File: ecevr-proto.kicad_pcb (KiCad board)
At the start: 4 copper layers, 100 x 92 mm, 359 parts, among them J1 CUR_SEL, J19 SFP, J2 PEN_SEL, J20 SFP_CAGE, J2001 BNC, J2051 BNC, J2201 BEL_0845_2G1T_H5, J3 USB_C_Receptacle_USB2.0, J4 JTAG, Q1 SSM6N35AFE, Q2 SSM6N35AFE, Q3 Si3477, SW1 PROG, SW2101 SW_DIP_x08, U1 XC7A35T-CSG325, U10 74VHC1G03, U11 UTC2000, U12 5P49V6965, U13 TPS3808DBV, U14 74LVC1G06, U15 74LVC2T45DC, U16 74LVC2T45DC, U2 AT25SL641, U2001 74LVC2T45DC, U2051 74LVC2T45DC, U2101 74AHC1T86, U2102 74AHC1T86, U2103 PCA9306, U2104 24AA0x, U2105 74AHC1T86, U2106 74AHC1T86, U2201 74AHC1T86, U2202 74LVC1G06, U2301 lan9254, U2302 SN74LV1T34DBV, U3 FT240XQ, U4 TLV62569ADDC, U5 TPS62A01A-SOT563, U6 TPS62A01A-SOT563, U7 TLV62569ADDC, U8 74ALVC125, U9 TLV62569ADDC, X2301 FNETHE025, Y1 25MHz

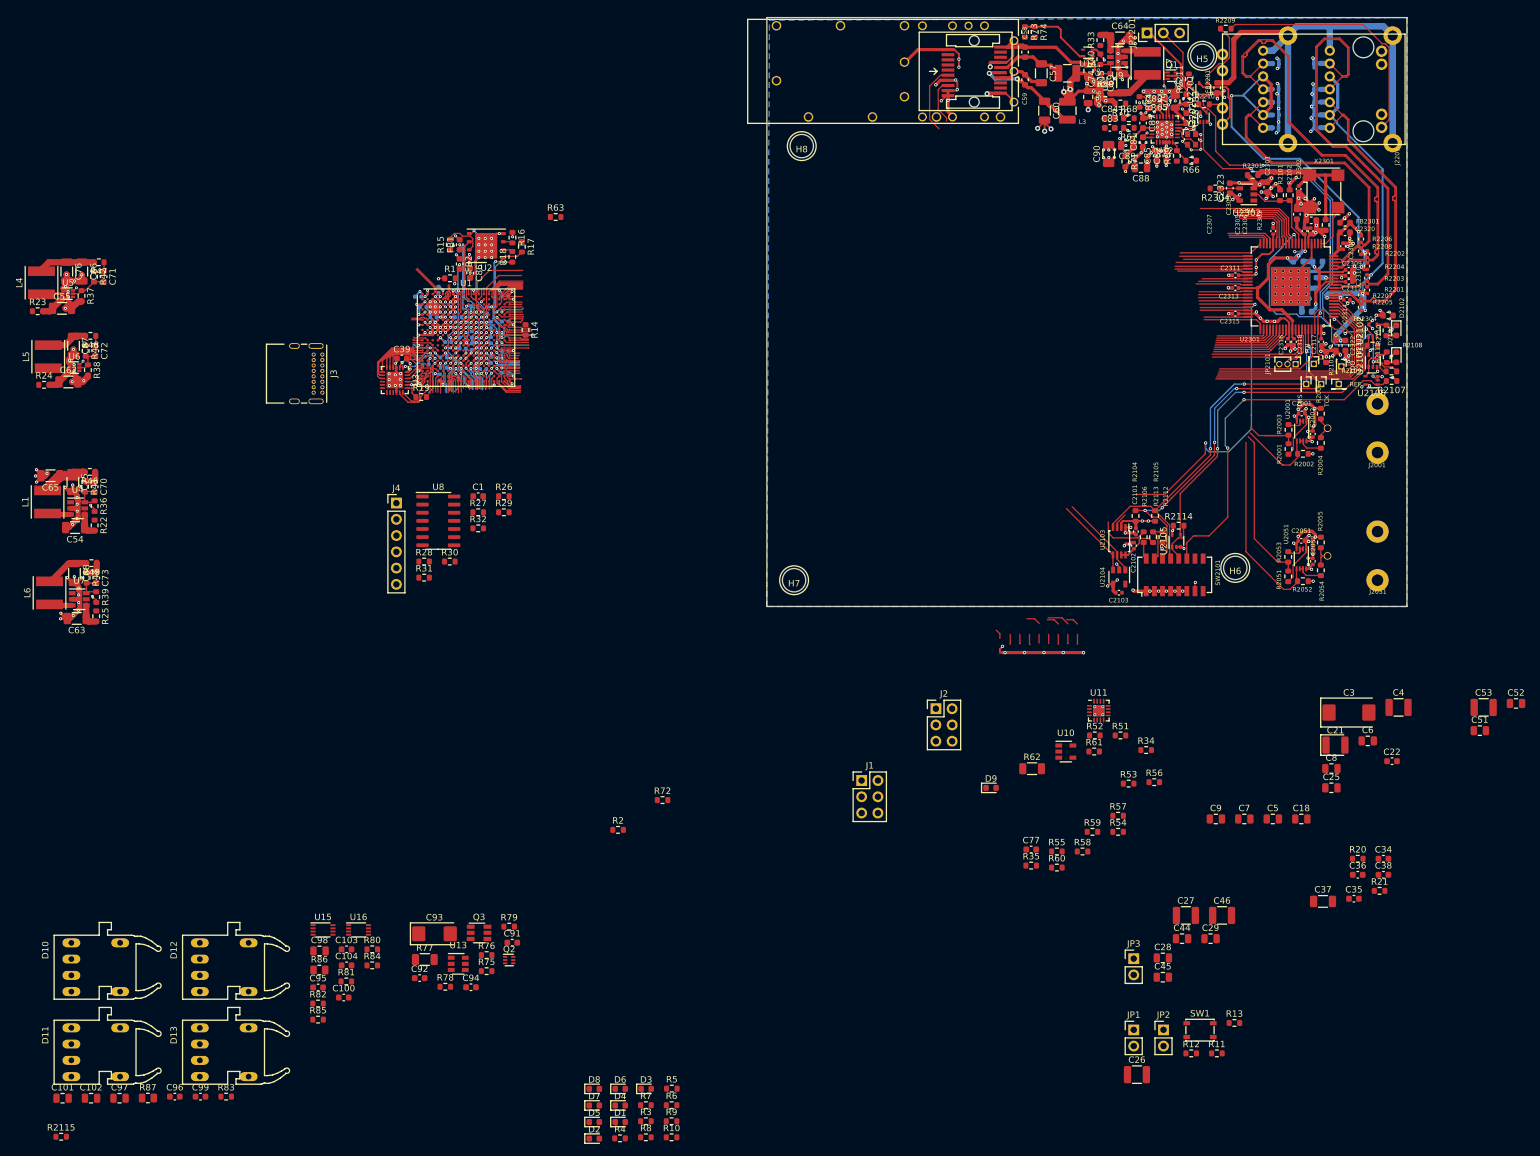
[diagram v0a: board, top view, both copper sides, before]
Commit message: further work...
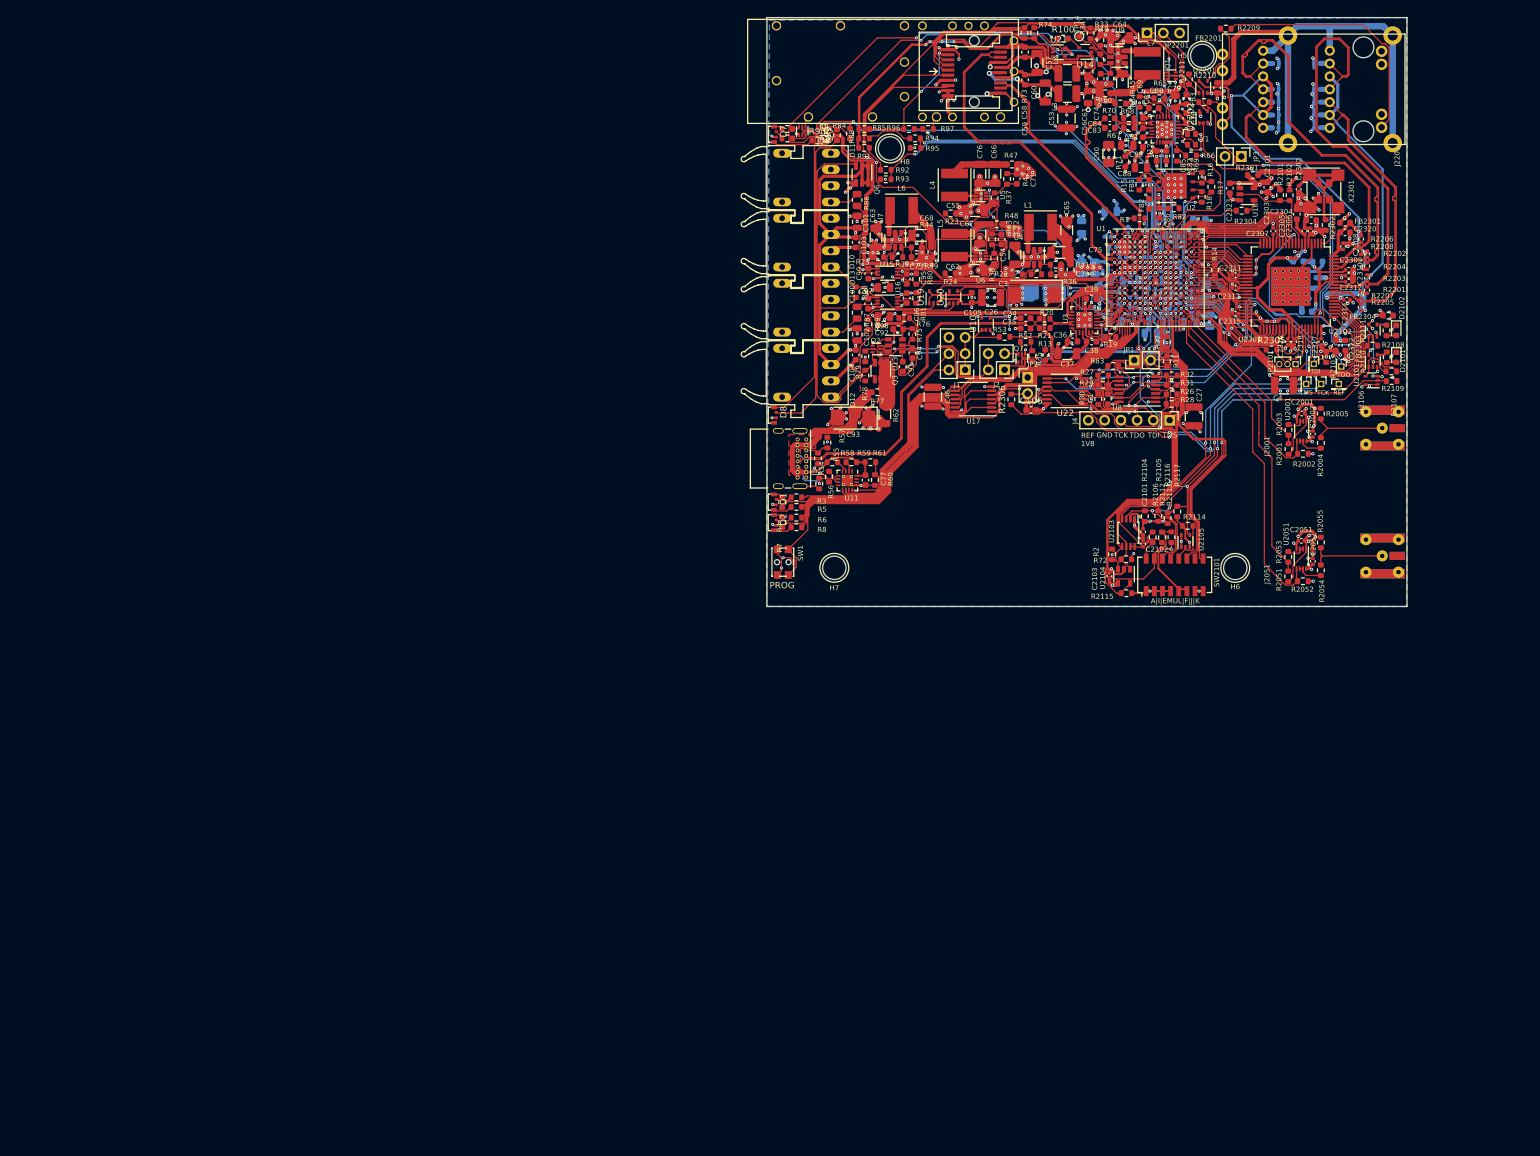
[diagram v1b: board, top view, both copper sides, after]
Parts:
- removed D3, D4, D5, D6, D9: LED, LED_SMD:LED_0603_1608Metric
- removed R51: 1k, Resistor_SMD:R_0603_1608Metric
- removed R63: 4k7, Resistor_SMD:R_0603_1608Metric
- removed U2302: SN74LV1T34DBV, Package_TO_SOT_SMD:SOT-23-5
- added C105: 100nF, Capacitor_SMD:C_0603_1608Metric, F.Cu at (132.0, 73.8)
- added C106: 100nF_603, Capacitor_SMD:C_0603_1608Metric, F.Cu at (141.3, 91.3)
- added Q4: SSM6N35AFE, proj_footprints:SOT-563-adjusted, F.Cu at (108.9, 47.5)
- added Q5: SSM6N35AFE, proj_footprints:SOT-563-adjusted, F.Cu at (105.5, 47.7)
- added Q6: Si3477, Package_TO_SOT_SMD:TSOT-23-6, F.Cu at (114.9, 54.5)
- added Q7: SSM6N35AFE, proj_footprints:SOT-563-adjusted, F.Cu at (139.8, 83.2)
- added R100: 2k, Resistor_SMD:R_0603_1608Metric, F.Cu at (146.3, 33.3)
- added R2116: 0, Resistor_SMD:R_0603_1608Metric, F.Cu at (162.6, 108.2)
- added R2117: 0, Resistor_SMD:R_0603_1608Metric, F.Cu at (164.1, 107.2)
- added R2305: 0, Resistor_SMD:R_0603_1608Metric, F.Cu at (178.8, 81.8)
- added R2306: 10k, Resistor_SMD:R_0603_1608Metric, F.Cu at (138.2, 89.7)
- added R88: 4k7, Resistor_SMD:R_0603_1608Metric, F.Cu at (115.2, 48.9)
- added R89: 1k, Resistor_SMD:R_0603_1608Metric, F.Cu at (115.8, 77.9)
- added R90: 1k, Resistor_SMD:R_0603_1608Metric, F.Cu at (113.9, 72.9)
- added R91: 4k7, Resistor_SMD:R_0603_1608Metric, F.Cu at (115.2, 50.4)
- added R92: 47k, Resistor_SMD:R_0603_1608Metric, F.Cu at (118.6, 53.8)
- added R93: 47k, Resistor_SMD:R_0603_1608Metric, F.Cu at (118.6, 55.3)
- added R94: 47k, Resistor_SMD:R_0603_1608Metric, F.Cu at (123.2, 48.9)
- added R95: 47k, Resistor_SMD:R_0603_1608Metric, F.Cu at (123.2, 50.4)
- added R96: 47k, Resistor_SMD:R_0603_1608Metric, F.Cu at (122.2, 47.4)
- added R97: 47k, Resistor_SMD:R_0603_1608Metric, F.Cu at (125.2, 47.4)
- added R98: 230, Resistor_SMD:R_0603_1608Metric, F.Cu at (107.9, 49.2)
- added R99: 750, Resistor_SMD:R_0603_1608Metric, F.Cu at (110.9, 48.4)
- added TP1: Dummy End, proj_footprints:endpoint_0.1mm, B.Cu at (162.8, 62.8)
- added TP10: Dummy End, proj_footprints:endpoint_0.1mm, F.Cu at (155.1, 79.4)
- added TP11: Dummy End, proj_footprints:endpoint_0.1mm, B.Cu at (157.5, 79.0)
- added TP12: Dummy End, proj_footprints:endpoint_0.1mm, B.Cu at (157.7, 79.0)
- added TP13: Dummy End, proj_footprints:endpoint_0.1mm, B.Cu at (157.9, 79.0)
- added TP14: TestPoint, TestPoint:TestPoint_Pad_D1.0mm, F.Cu at (148.8, 32.9)
- added TP2: Dummy End, proj_footprints:endpoint_0.1mm, F.Cu at (163.1, 62.8)
- added TP3: Dummy End, proj_footprints:endpoint_0.1mm, B.Cu at (164.8, 62.3)
- added TP4: Dummy End, proj_footprints:endpoint_0.1mm, B.Cu at (164.4, 79.0)
- added TP5: Dummy End, proj_footprints:endpoint_0.1mm, F.Cu at (164.8, 79.0)
- added TP6: Dummy End, proj_footprints:endpoint_0.1mm, B.Cu at (163.9, 79.0)
- added TP7: Dummy End, proj_footprints:endpoint_0.1mm, F.Cu at (163.9, 79.0)
- added TP8: Dummy End, proj_footprints:endpoint_0.1mm, F.Cu at (164.3, 79.0)
- added U17: 74LVC06, Package_SO:TSSOP-14_4.4x5mm_P0.65mm, F.Cu at (132.3, 89.6)
- added U18: 74LVC1T126, Package_TO_SOT_SMD:SOT-23-5, F.Cu at (175.0, 57.6)
- added U19: 74AHC1T86, Package_TO_SOT_SMD:SOT-353_SC-70-5, F.Cu at (126.0, 73.7)
- added U20: 74AHC1T86, Package_TO_SOT_SMD:SOT-353_SC-70-5, F.Cu at (129.1, 73.7)
- added U21: 74LVC1G06, Package_TO_SOT_SMD:SOT-353_SC-70-5, F.Cu at (145.6, 35.4)
- added U22: 74AC126, Package_SO:TSSOP-14_4.4x5mm_P0.65mm, F.Cu at (146.6, 88.3)
- C18, C21, C25, C28, C29, C44, C45, C5, C51, C52, C6, C7, C8, C9: moved to B.Cu
- C22: footprint Capacitor_SMD:C_0603_1608Metric -> Capacitor_SMD:C_0402_1005Metric; moved to B.Cu
- D1, D2, D7, D8: value LED -> LED_BARG; footprint LED_SMD:LED_0603_1608Metric -> proj_footprints:LED_RGB_2504_horiz_barg
- J2: footprint Connector_PinHeader_2.54mm:PinHeader_2x03_P2.54mm_Vertical -> Connector_PinHeader_2.54mm:PinHeader_2x02_P2.54mm_Vertical
- J2001, J2051: footprint proj_footprints:BNC_Molex_0731713150 -> proj_footprints:LEMO+SMA
- R10, R3, R6: value 1k -> 750
- R15, R16, R17: value 2k4 -> 10k
- R2002, R2052: value 2k2 -> 3k3
- R2108: value 1k -> 10k
- R2110: value 100 -> 1k5
- R2111: value 100 -> 3k3
- R22, R23, R24, R25, R33: value 10k -> 100k
- R2209, R2210: value 100 -> 178
- R2211: value 100 -> 10k
- R4, R7, R9: value 1k -> 2k
- R40: value 45.9k -> 10k
- R45: value 10.2k -> 45k3
- R5, R8: value 1k -> 230
- R52, R76: value 100k -> 10k
- R66: value 1k78 -> 10k
- R75: value 100k -> 45.3k
- R77: value 47 -> 50; footprint Resistor_SMD:R_1206_3216Metric -> Resistor_SMD:R_0603_1608Metric
- R82, R83: value 1k -> 100k
- R84, R85: value 1k -> 4k7
- R86, R87: value 90 -> 100
- SW1: footprint Button_Switch_SMD:SW_SPST_PTS810 -> proj_footprints:SW_SPST_PTS810_and_PTS841
- U10: value 74VHC1G03 -> 74LVC1G06; footprint Package_TO_SOT_SMD:SOT-23-5 -> Package_TO_SOT_SMD:SOT-353_SC-70-5
- U14, U2202: footprint proj_footprints:SOT-5x3 -> Package_TO_SOT_SMD:SOT-353_SC-70-5
- U2104: value 24AA0x -> 24FC16T
- U8: footprint Package_SO:SOIC-14_3.9x8.7mm_P1.27mm -> Package_SO:TSSOP-14_4.4x5mm_P0.65mm
- X2301: footprint Oscillator:Oscillator_SMD_Diodes_FN-4Pin_7.0x5.0mm -> proj_footprints:FNETH_and_ASE-4Pin_3.2x2.5mm
- moved R2115 186.8 mm to (156.2, 119.9)
- moved C101 184.8 mm to (114.1, 61.9), turned to 90 degrees
- moved R82 182.5 mm to (163.6, 59.8)
- moved D11 181.0 mm to (110.0, 55.0), turned to 180 degrees
- moved R83 179.5 mm to (154.1, 84.4)
- moved C97 174.1 mm to (118.3, 72.2)
- moved C96 169.2 mm to (121.8, 73.8), turned to 90 degrees
- moved C102 169.0 mm to (114.1, 79.5), turned to 90 degrees
- moved C99 165.6 mm to (115.8, 70.0), turned to 90 degrees
- moved R87 165.3 mm to (114.1, 76.1), turned to 270 degrees
- moved D10 164.0 mm to (110.0, 65.2), turned to 180 degrees
- moved C65 163.3 mm to (146.8, 63.2), turned to 90 degrees
- moved R85 163.2 mm to (115.2, 47.4), turned to 180 degrees
- moved L1 161.0 mm to (142.8, 62.8), turned to 0 degrees
- moved C75 158.4 mm to (145.9, 66.7), turned to 180 degrees
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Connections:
- C101 pad 1: +5V -> +5V_SWITCHED
- C102 pad 1: +5V -> +5V_SWITCHED
- C103 pad 2: +5V -> +5V_SWITCHED
- C104 pad 2: +5V -> +5V_SWITCHED
- D1 pad 1: GND -> Net-(D1-Pad1)
- D1 pad 2: Net-(D1-Pad2) -> +5V
- D10 pad 3: +5V -> +5V_SWITCHED
- D12 pad 3: +5V -> +5V_SWITCHED
- D2 pad 1: GND -> Net-(D2-Pad1)
- D2 pad 2: Net-(D2-Pad2) -> +5V
- D7 pad 1: GND -> Net-(D7-Pad1)
- D7 pad 2: Net-(D7-Pad2) -> +5V
- D8 pad 1: GND -> Net-(D8-Pad1)
- D8 pad 2: Net-(D8-Pad2) -> +5V
- J19 pad 2: IO_L7N_T1_AD2N_15 -> Net-(J19-Pad2)
- J19 pad 6: IO_L5N_T0_AD9N_15 -> Net-(J19-Pad6)
- J19 pad 8: IO_L4N_T0_15 -> Net-(J19-Pad8)
- J2 pad 2: USB_BCDb -> Net-(J2-Pad2)
- J2 pad 3: Net-(J2-Pad1) -> Net-(J2-Pad3)
- J2 pad 4: IO_L15N_T2_DQS_34 -> Net-(J2-Pad2)
- Q1 pad 1: IO_L7P_T1_AD2P_15 -> IO_L4N_T0_15
- Q2 pad 3: Net-(Q2-Pad3) -> Net-(J2-Pad2)
- R10 pad 1: IO_L20P_T3_34 -> Net-(D7-Pad3)
- R10 pad 2: Net-(D8-Pad2) -> Net-(Q5-Pad3)
- R2 pad 2: IO_L23N_T3_A02_D18_14 -> IO_L23P_T3_A03_D19_14
- R2107 pad 1: +3V3 -> GND
- R2108 pad 2: Net-(R2108-Pad2) -> IO_L22P_T3_A05_D21_14
- R2112 pad 1: IO_L21P_T3_DQS_14 -> IO_L23N_T3_A02_D18_14
- R2113 pad 2: IO_L21P_T3_DQS_14 -> IO_L23N_T3_A02_D18_14
- R2114 pad 1: +1V8 -> GND
- R2114 pad 2: IO_L22P_T3_A05_D21_14 -> Net-(R2114-Pad2)
- R3 pad 1: IO_L3P_T0_DQS_34 -> Net-(R3-Pad1)
- R3 pad 2: Net-(D1-Pad2) -> Net-(D1-Pad3)
- R35 pad 1: Net-(R35-Pad1) -> USB_BCDb
- R35 pad 2: +5V -> GND
- R4 pad 1: IO_L3N_T0_DQS_34 -> Net-(R4-Pad1)
- R4 pad 2: Net-(D2-Pad2) -> Net-(D1-Pad4)
- R5 pad 1: IO_L18N_T2_34 -> Net-(R5-Pad1)
- R5 pad 2: Net-(D3-Pad2) -> Net-(D1-Pad1)
- R52 pad 1: Net-(J2-Pad1) -> IO_L15N_T2_DQS_34
- R52 pad 2: +5V -> GND
- R6 pad 1: IO_L18P_T2_34 -> Net-(R6-Pad1)
- R6 pad 2: Net-(D4-Pad2) -> Net-(D2-Pad3)
- R64 pad 1: IO_L7P_T1_AD2P_15 -> IO_L4N_T0_15
- R7 pad 1: IO_25_34 -> Net-(R7-Pad1)
- R7 pad 2: Net-(D5-Pad2) -> Net-(D2-Pad4)
- R72 pad 2: IO_L23P_T3_A03_D19_14 -> IO_L21P_T3_DQS_14
- R8 pad 1: IO_L20N_T3_34 -> Net-(R8-Pad1)
- R8 pad 2: Net-(D6-Pad2) -> Net-(D2-Pad1)
- R80 pad 1: IO_L22P_T3_34 -> IO_L4P_T0_34
- R81 pad 1: IO_L22N_T3_34 -> IO_L4N_T0_34
- R82 pad 1: IO_L24N_T3_34 -> +1V8
- R82 pad 2: GND -> Net-(R82-Pad2)
- R83 pad 1: IO_L24P_T3_34 -> +1V8
- R83 pad 2: GND -> TDO
- R84 pad 1: IO_L24N_T3_34 -> /CFG_DONE
- R84 pad 2: Net-(D10-Pad1) -> +1V8
- R85 pad 1: IO_L24P_T3_34 -> Net-(J19-Pad2)
- R85 pad 2: Net-(D12-Pad1) -> +3V3
- R9 pad 1: IO_L23N_T3_34 -> Net-(D7-Pad4)
- R9 pad 2: Net-(D7-Pad2) -> Net-(Q5-Pad6)
- SW1 pad 1: Net-(R12-Pad1) -> GND
- SW1 pad 2: GND -> Net-(R12-Pad1)
- SW2101 pad 10: IO_L21N_T3_DQS_A06_D22_14 -> IO_L22N_T3_A04_D20_14
- SW2101 pad 12: IO_L22P_T3_A05_D21_14 -> Net-(R2114-Pad2)
- SW2101 pad 15: IO_L21P_T3_DQS_14 -> IO_L23N_T3_A02_D18_14
- SW2101 pad 5: GND -> +1V8
- SW2101 pad 6: GND -> +1V8
- SW2101 pad 9: IO_L22N_T3_A04_D20_14 -> IO_L21N_T3_DQS_A06_D22_14
- U1 pad F12: Net-(R63-Pad1) -> /CFG_DONE
- U1 pad K16: Net-(U1-PadK16) -> Net-(R82-Pad2)
- U10 pad 2: Net-(J2-Pad1) -> Net-(J1-Pad1)
- U12 pad 9: IO_L7P_T1_AD2P_15 -> IO_L4N_T0_15
- U13 pad 3: Net-(Q2-Pad3) -> Net-(J2-Pad2)
- U14 pad 1: Net-(U14-Pad1) -> +3V3
- U14 pad 2: IO_L5P_T0_AD9P_15 -> +3V3
- U14 pad 4: /SFP Connector/TX_DISABLE -> Net-(R100-Pad2)
- U15 pad 6: IO_L22P_T3_34 -> IO_L4P_T0_34
- U15 pad 7: IO_L22P_T3_34 -> IO_L4P_T0_34
- U16 pad 6: IO_L22N_T3_34 -> IO_L4N_T0_34
- U16 pad 7: IO_L22N_T3_34 -> IO_L4N_T0_34
- U2 pad 5: Net-(U1-PadK16) -> Net-(R82-Pad2)
- U2102 pad 1: Net-(R2108-Pad2) -> IO_L22P_T3_A05_D21_14
- U2103 pad 5: IO_L23N_T3_A02_D18_14 -> IO_L23P_T3_A03_D19_14
- U2103 pad 6: IO_L23P_T3_A03_D19_14 -> IO_L21P_T3_DQS_14
- U2104 pad 1: IO_L23P_T3_A03_D19_14 -> IO_L21P_T3_DQS_14
- U2104 pad 3: IO_L23N_T3_A02_D18_14 -> IO_L23P_T3_A03_D19_14
- U2105 pad 1: IO_L22P_T3_A05_D21_14 -> +1V8
- U2105 pad 2: GND -> Net-(R2114-Pad2)
- U2105 pad 4: Net-(R2108-Pad2) -> IO_L22P_T3_A05_D21_14
- U2106 pad 1: Net-(R2107-Pad2) -> +3V3
- U2106 pad 2: GND -> Net-(R2107-Pad2)
- U2202 pad 1: Net-(U2202-Pad1) -> /lan9254/LINKACT1
- U2301 pad 41: IO_L7P_T1_D09_14 -> IO_L7N_T1_D10_14
- U2301 pad 42: IO_L7N_T1_D10_14 -> IO_L7P_T1_D09_14
- U8 pad 13: GND -> /LAN9254_JTAG_EN
- U8 pad 2: TCK_I -> TMS_I
- U8 pad 3: TCK -> TMS
- U8 pad 5: TDI_I -> TCK_I
- U8 pad 6: TDI -> TCK
- U8 pad 8: TMS -> TDI
- U8 pad 9: TMS_I -> TDI_I
- U9 pad 5: Net-(R35-Pad1) -> Net-(TP14-Pad1)
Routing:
- net GND: track 511.4 -> 693.5 mm, vias 311 -> 392
- net +1V8: track 159.3 -> 333.8 mm, vias 74 -> 120
- net +5V: track 19.4 -> 133.1 mm, vias 0 -> 55
- net Net-(D8-Pad4): track 0.00 -> 101.5 mm, vias 0 -> 2
- net Net-(R12-Pad1): track 5.25 -> 99.5 mm, vias 1 -> 3
- net IO_L22P_T3_A05_D21_14: track 10.0 -> 93.1 mm, vias 1 -> 6
- net +5V_SWITCHED: track 0.00 -> 72.5 mm, vias 0 -> 4
- net Net-(R34-Pad2): track 0.00 -> 72.4 mm
- net /CFG_DONE: track 0.00 -> 72.1 mm, vias 0 -> 2
- net IO_L3P_T0_DQS_34: track 2.40 -> 74.3 mm
- net IO_L3N_T0_DQS_34: track 1.58 -> 72.4 mm
- net SDA1_3V3: track 0.86 -> 64.1 mm, vias 0 -> 2
- net +1V0: track 33.4 -> 96.1 mm, vias 22 -> 42
- net IO_L12P_T1_MRCC_34: track 5.67 -> 67.8 mm, vias 1 -> 4
- net /LAN9254_JTAG_EN: track 0.00 -> 61.8 mm, vias 0 -> 4
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- added copper zone on In2.Cu, net +5V
- added copper zone on F.Cu, net VBUS
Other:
- board text added: "A|I|EMUL|F|J|K"
- board text added: "EtherCat EVR V1.1.0"
- board text added: "GND"
- board text added: "REF 1V8"
- board text added: "TCK"
- board text added: "TDI"
- board text added: "TDO"
- board text added: "TMS"
- board text removed: "EtherCat / Zynq Development Board V1.0.0"
